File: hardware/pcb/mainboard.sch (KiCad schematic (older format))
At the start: 27 parts

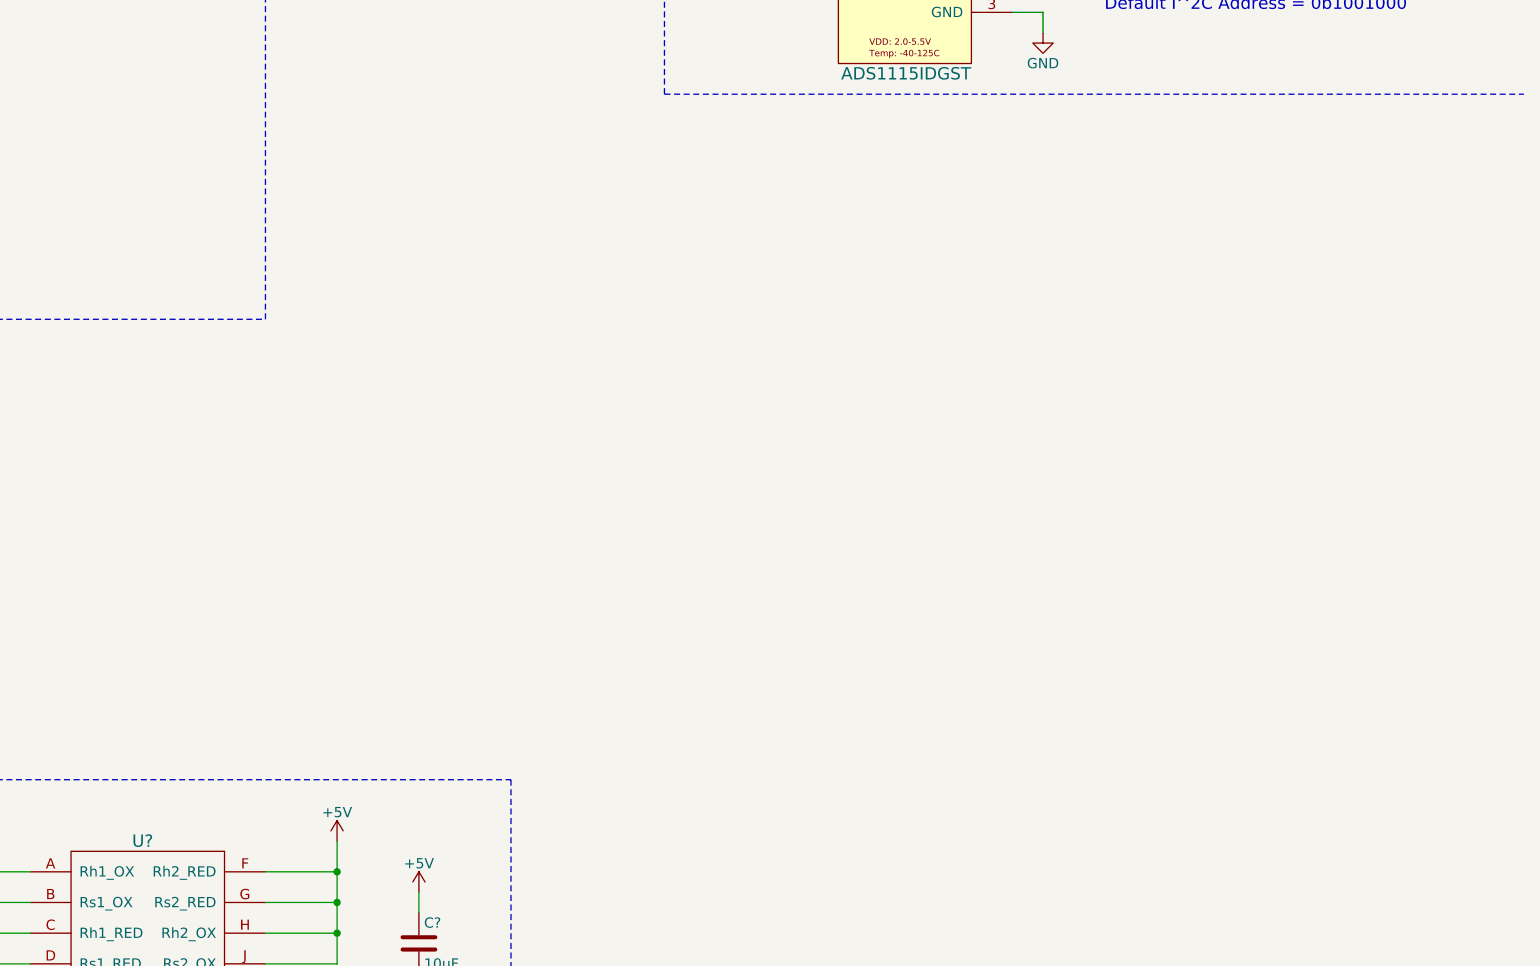
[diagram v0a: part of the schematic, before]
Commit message: Working on Radio and arm m0
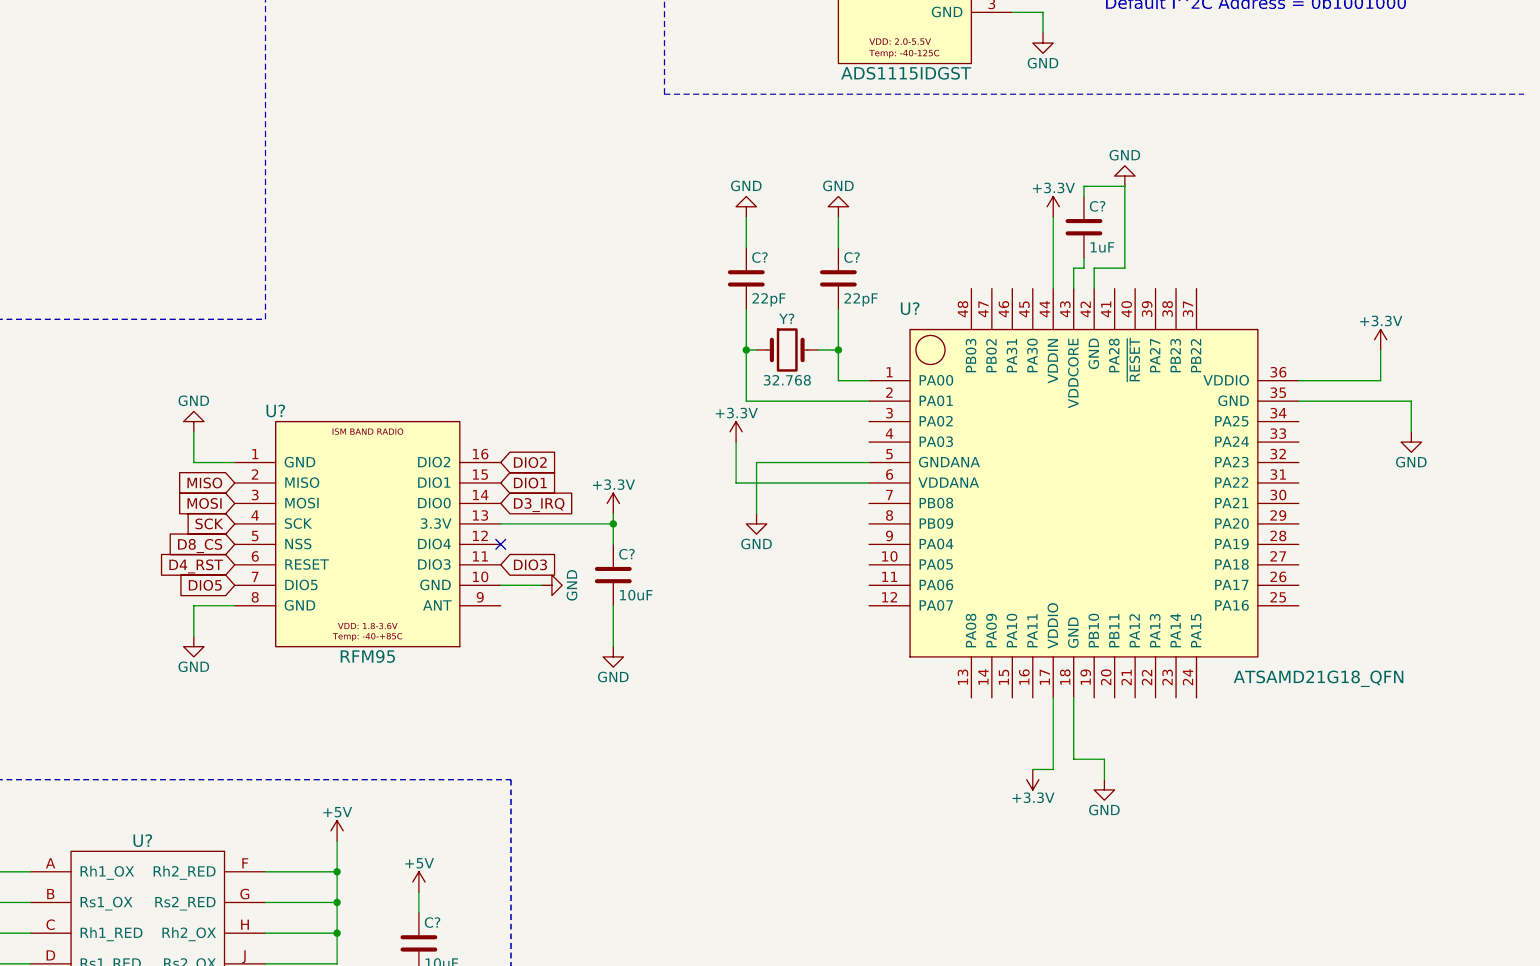
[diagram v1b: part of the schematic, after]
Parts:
- added C?: 1uF, symbol C
- added C? (x2): 22pF, symbol C
- added C?: 10uF, symbol C
- added U?: ATSAMD21G18_QFN, symbol ATSAMD21G18_QFN
- added U?: RFM95, symbol RFM95
- added Y?: 32.768, symbol Crystal
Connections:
- net +3V3: now also C?.1, U?.13 (3.3V), U?.17 (VDDIO), U?.36 (VDDIO), U?.44 (VDDIN), U?.6 (VDDANA)
- net GND: now also C?.1, C?.1, C?.1, C?.2, U?.1 (GND), U?.10 (GND), U?.18 (GND), U?.35 (GND), U?.42 (GND), U?.5 (GNDANA), U?.8 (GND)
- new net: C?.2, U?.1 (PA00), Y?.2
- new net: C?.2, U?.2 (PA01), Y?.1
- new net: C?.2, U?.43 (VDDCORE)
- new net D3_IRQ: U?.14 (DIO0)
- new net D4_RST: U?.6 (RESET)
- new net D8_CS: U?.5 (NSS)
- new net DIO1: U?.15 (DIO1)
- new net DIO2: U?.16 (DIO2)
- new net DIO3: U?.11 (DIO3)
- new net DIO5: U?.7 (DIO5)
- new net MISO: U?.2 (MISO)
- new net MOSI: U?.3 (MOSI)
- new net SCK: U?.4 (SCK)
- no-connect marks 2 -> 3
